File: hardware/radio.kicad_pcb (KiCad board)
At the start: 4 copper layers, 65 x 56 mm, 89 parts, among them J1 JCLK, U1 G144A12, U3V3t1V8 NCP1117ST18T3G, U5V0t3V3 NCP1117ST33T3G

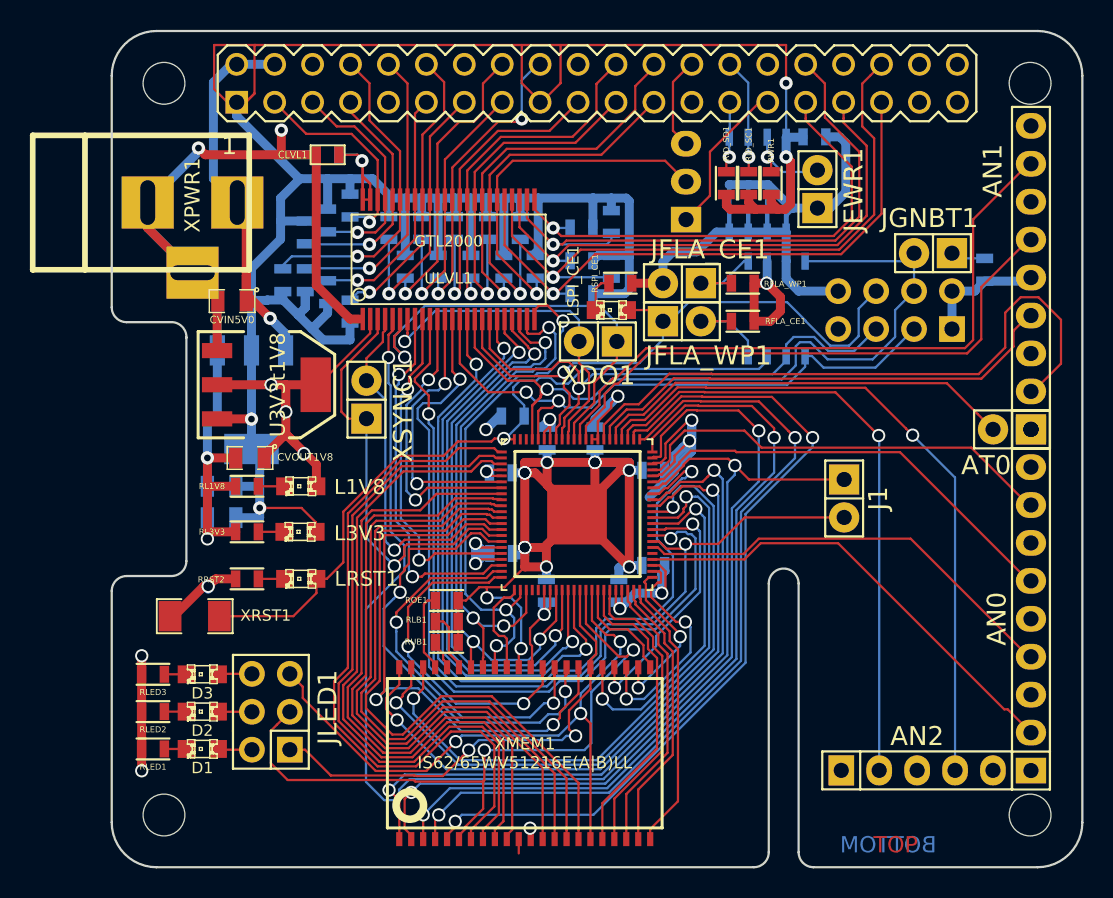
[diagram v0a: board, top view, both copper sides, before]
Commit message: More 4 layer work.
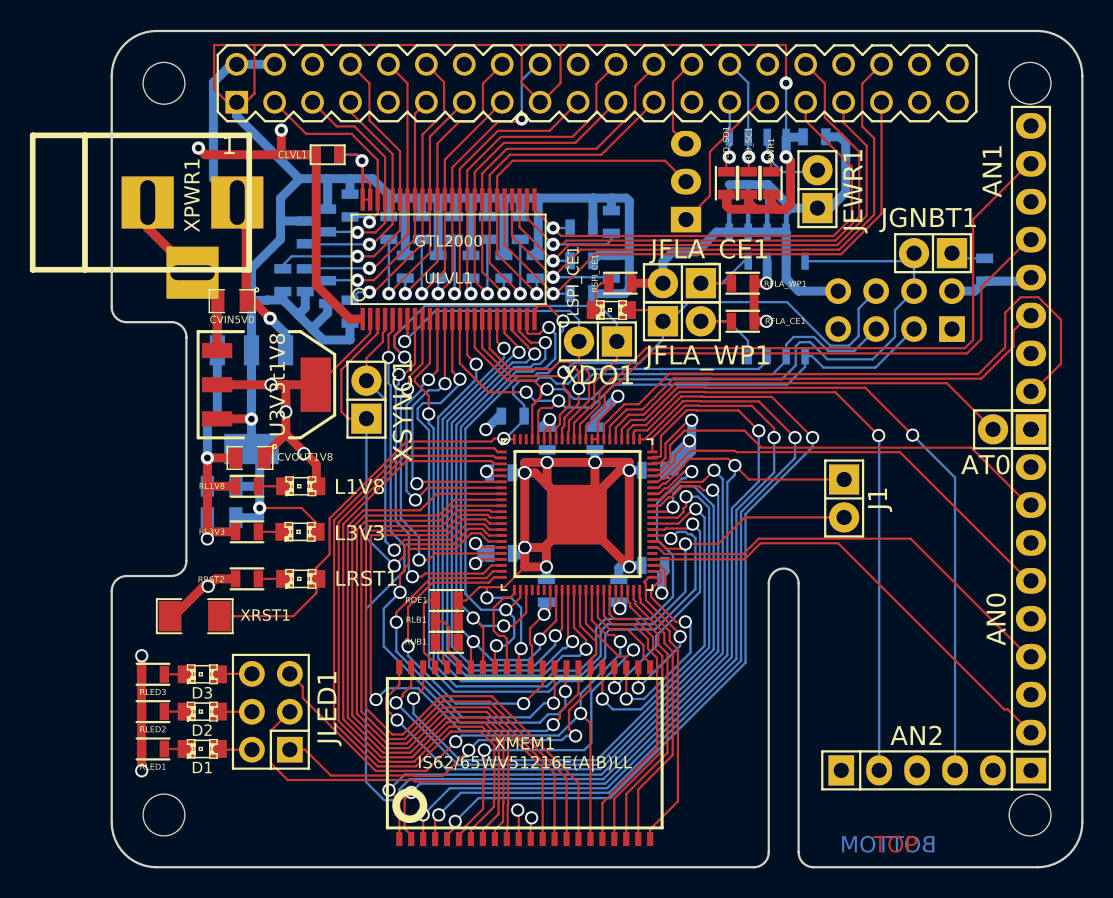
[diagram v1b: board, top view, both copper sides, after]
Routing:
- net GND: track 221.9 -> 447.5 mm
- net VDD: track 107.8 -> 232.0 mm, vias 15 -> 17
- net +3.3V: track 203.8 -> 202.6 mm
- net /DATA8: track 37.7 -> 38.5 mm
